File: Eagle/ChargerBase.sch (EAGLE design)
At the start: 51 parts, among them IC1 NE5532D, IC2 TINY24/44/84-SSU, IC3 NE5532D, Q1 2N3906, Q2 2N3906, Q3 2N3906, T1 2N3904, T2 2N3904, T3 2N3904, T4 2N3904

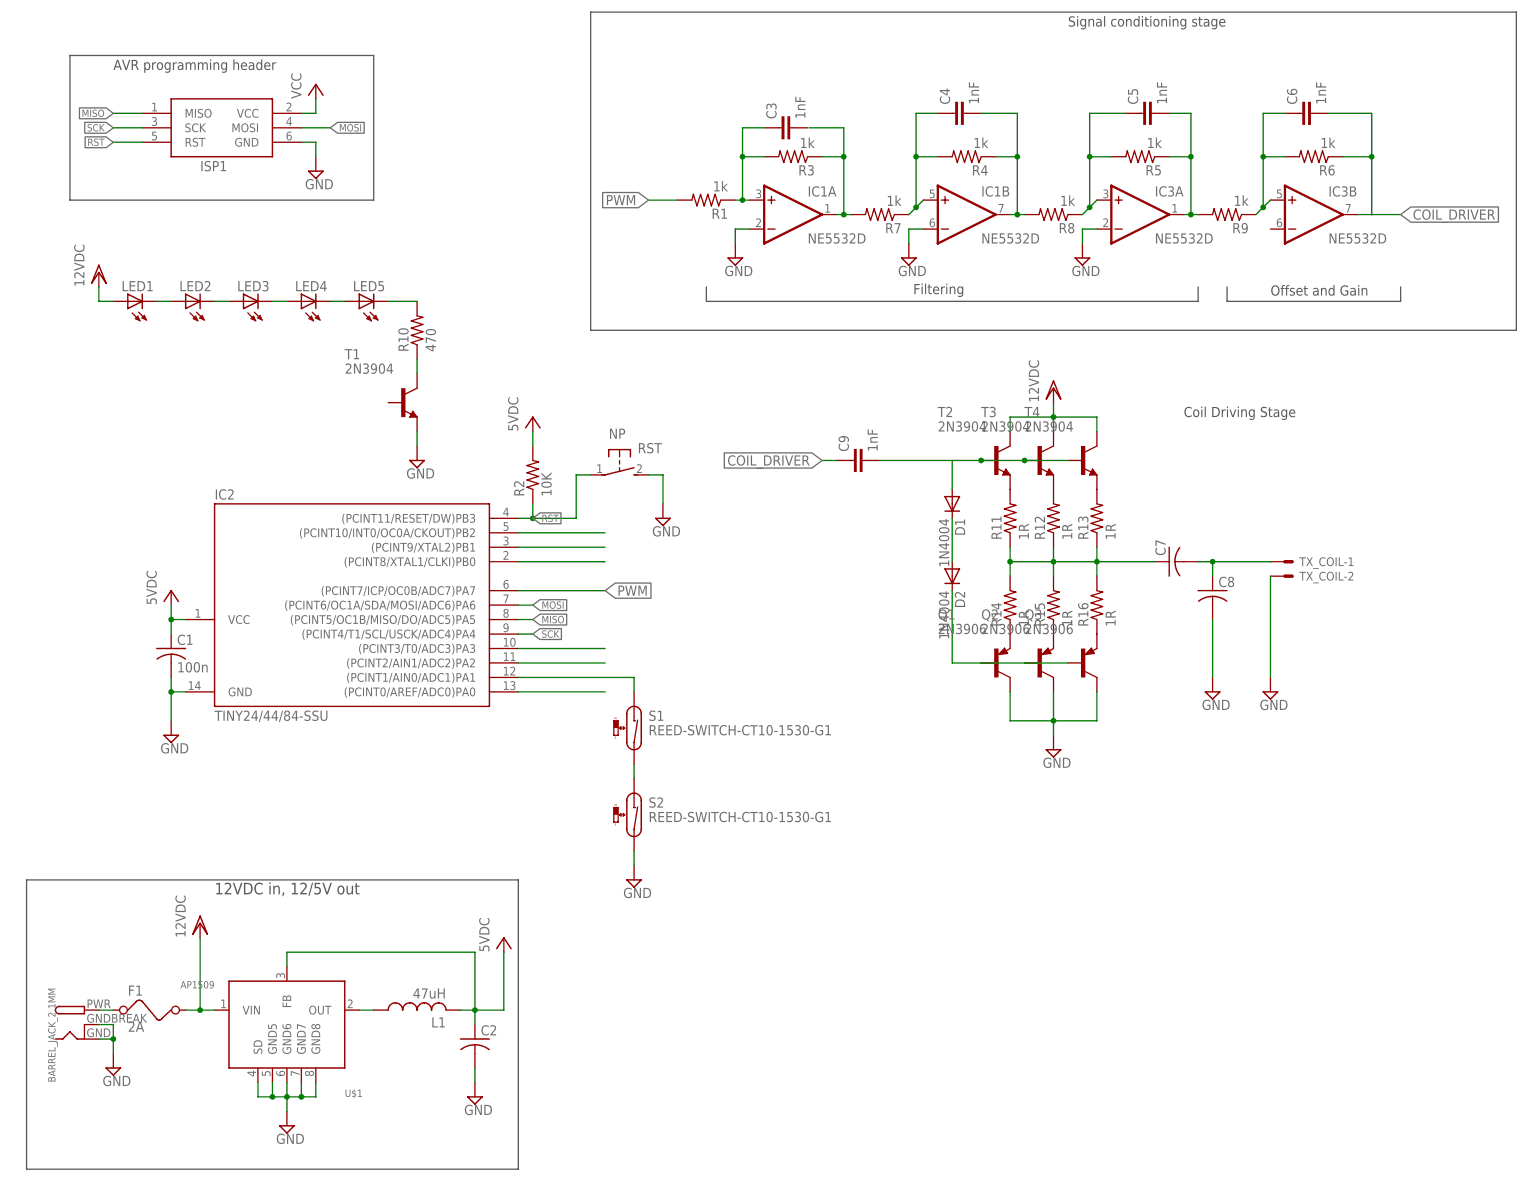
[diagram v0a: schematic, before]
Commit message: Uploaded schematics
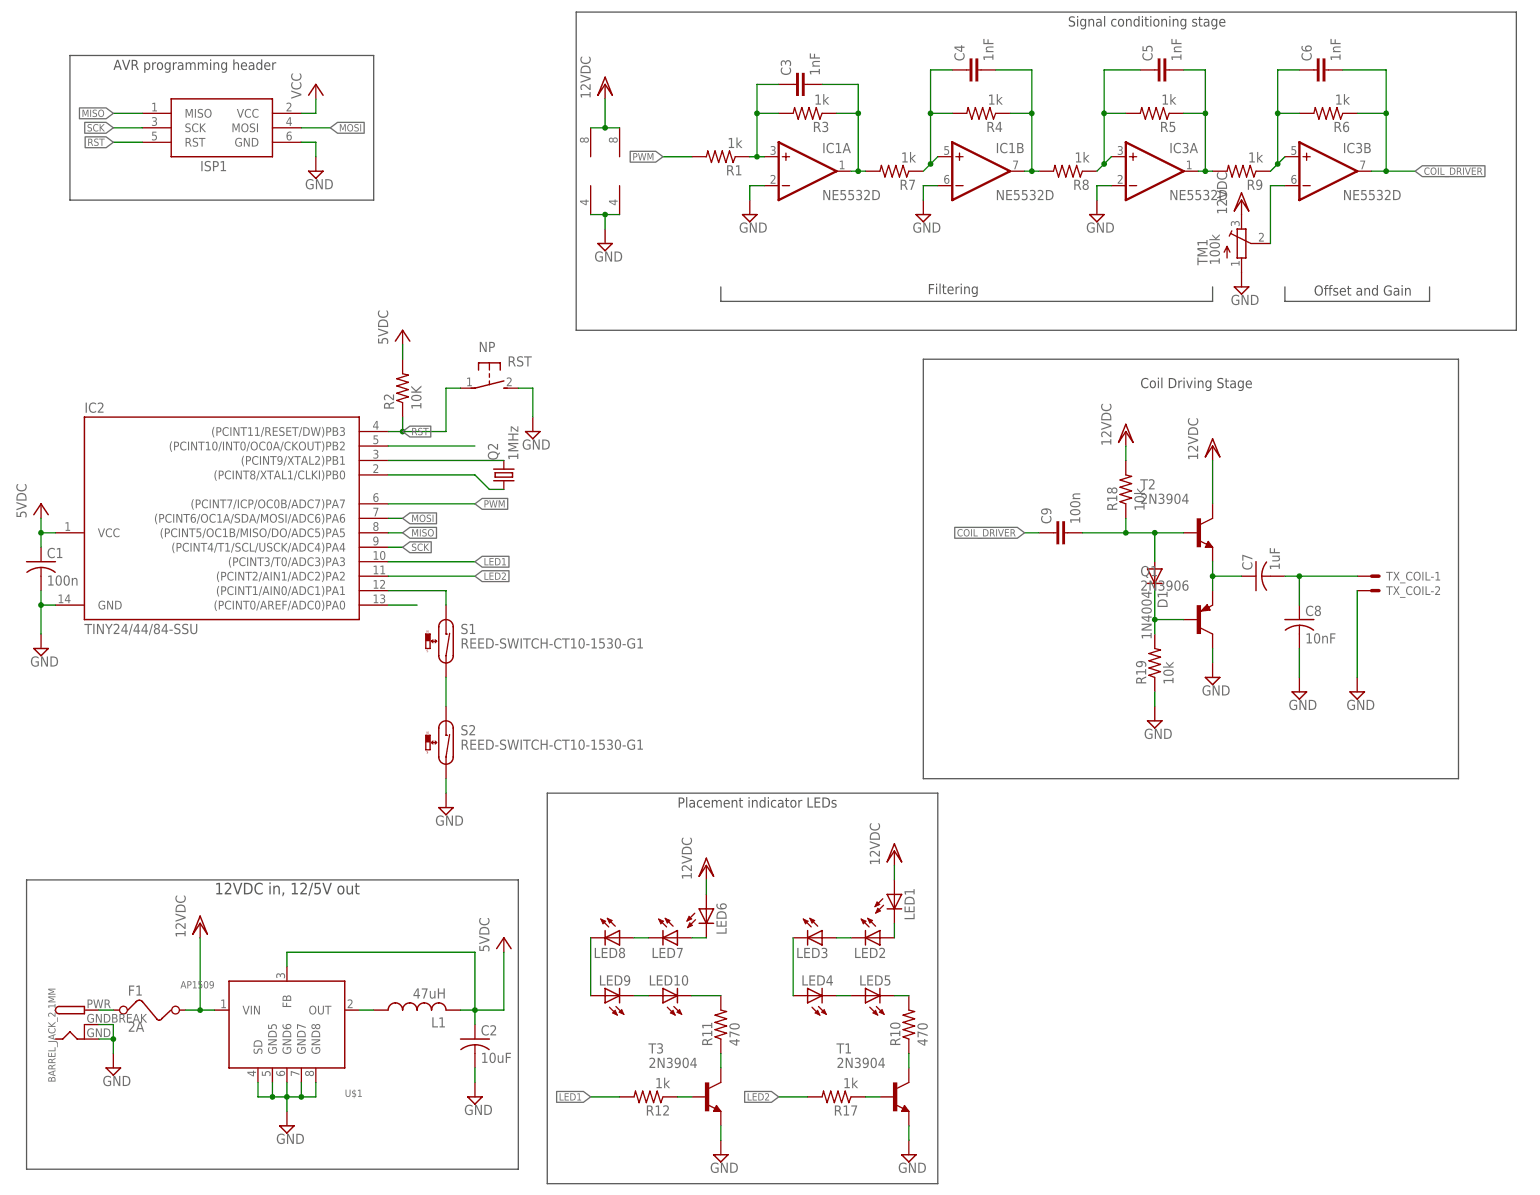
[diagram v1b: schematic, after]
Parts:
- removed D2: 1N4004, adafruit:1N4004
- removed Q3: 2N3906, transistor-pnp:2N3906
- removed R13, R14, R15, R16: 1R, rcl:R-US_R0805
- removed T4: 2N3904, transistor:2N3904
- added LED10, LED6, LED7, LED8, LED9: (no value), led:LEDCHIPLED_0805
- added R17: 1k, rcl:R-US_R0805
- added R18, R19: 10k, rcl:R-US_R0805
- added TM1: 100k, adafruit:TRIMPOTTC33X
- C2: value (none) -> 10uF
- C7: value (none) -> 1uF
- C8: value (none) -> 10nF
- C9: value 1nF -> 100n
- Q2: value 2N3906 -> 1MHz; device transistor-pnp:2N3906 -> adafruit:CRYSTALSM49
- R11: value 1R -> 470
- R12: value 1R -> 1k
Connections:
- removed net N$23: R13.2, T4.E
- removed net PIN10: IC2.(PCINT3/T0/ADC3)PA3
- removed net PIN11: IC2.(PCINT2/AIN1/ADC2)PA2
- new net LED1: IC2.(PCINT3/T0/ADC3)PA3, R12.2
- new net LED2: IC2.(PCINT2/AIN1/ADC2)PA2, R17.2
- new net N$14: R17.1, T1.B
- new net N$32: R11.1, T3.C
- new net N$33: R12.1, T3.B
- net GND: now also IC1P.V-, IC3P.V-, R19.1, T3.E, TM1.A; no longer Q2.C, Q3.C
- net N$15: now also IC3B.-IN, TM1.S; no longer R12.2, T3.E
- net N$16: now also T1.C
- net N$24: now also LED7.C, LED8.A; no longer Q1.E, R14.1
- net N$25: now also LED8.C, LED9.A; no longer Q2.E, R15.1
- net N$26: now also LED10.A, LED9.C; no longer Q3.E, R16.1
- net N$27: now also Q1.E, T2.E; no longer R11.1, R12.1, R13.1, R14.2, R15.2, R16.2
- net N$28: now also R18.1; no longer T3.B, T4.B
- net N$29: now also Q1.B, R19.2; no longer D2.A
- net N$3: now also Q2.1
- net N$31: now also LED10.C, R11.2; no longer D2.C, Q1.B, Q2.B, Q3.B
- net N$4: now also Q2.2
- net N$6: now also LED6.C, LED7.A; no longer R11.2, T2.E
- net N$8: now also C3.2
- net VDD: now also IC1P.V+, IC3P.V+, LED6.A, R18.2, TM1.E; no longer T3.C, T4.C
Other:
- note added: "Placement indicator LEDs"
- moved on the sheet: C1, C3, C4, C5, C6, C7, C8, C9, D1, IC1A, IC1B, IC2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
